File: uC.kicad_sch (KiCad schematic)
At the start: 21 parts, among them J7 Conn_01x03, P12 Conn_02x10_Odd_Even, SW1 SW_MEC_5E, SW2 SW_MEC_5E, U1 RPi-Pico

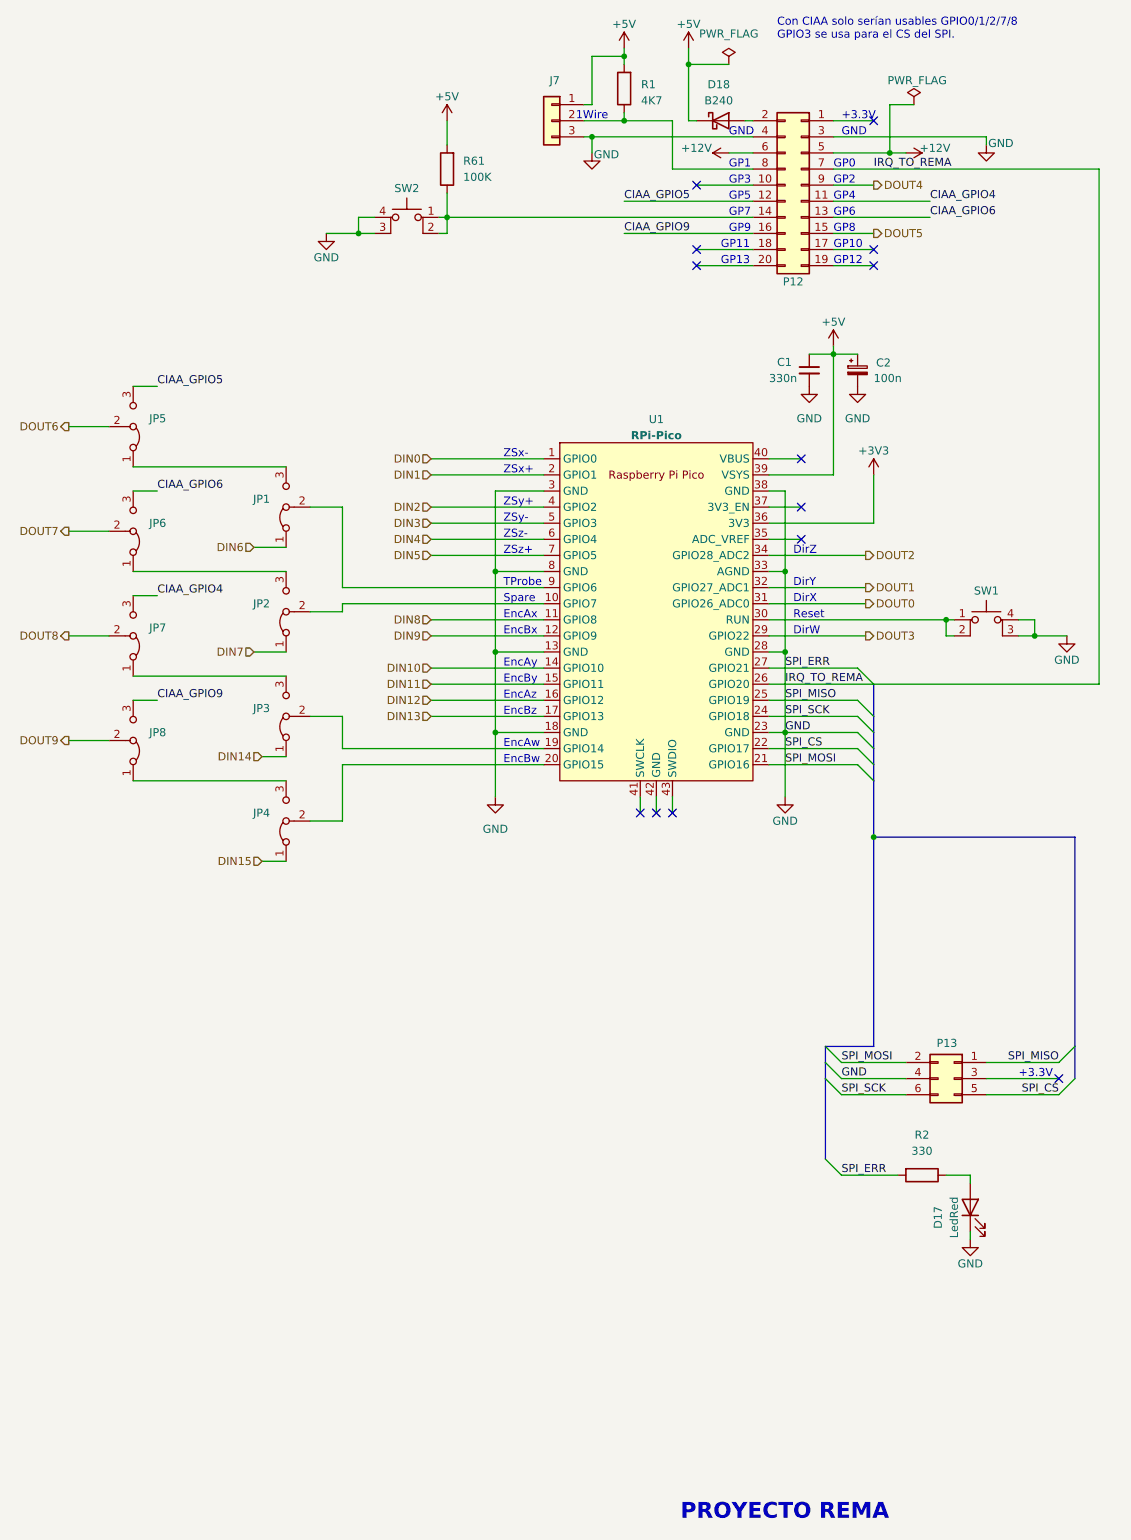
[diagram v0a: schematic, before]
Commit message: Comienza el diseño del pcb
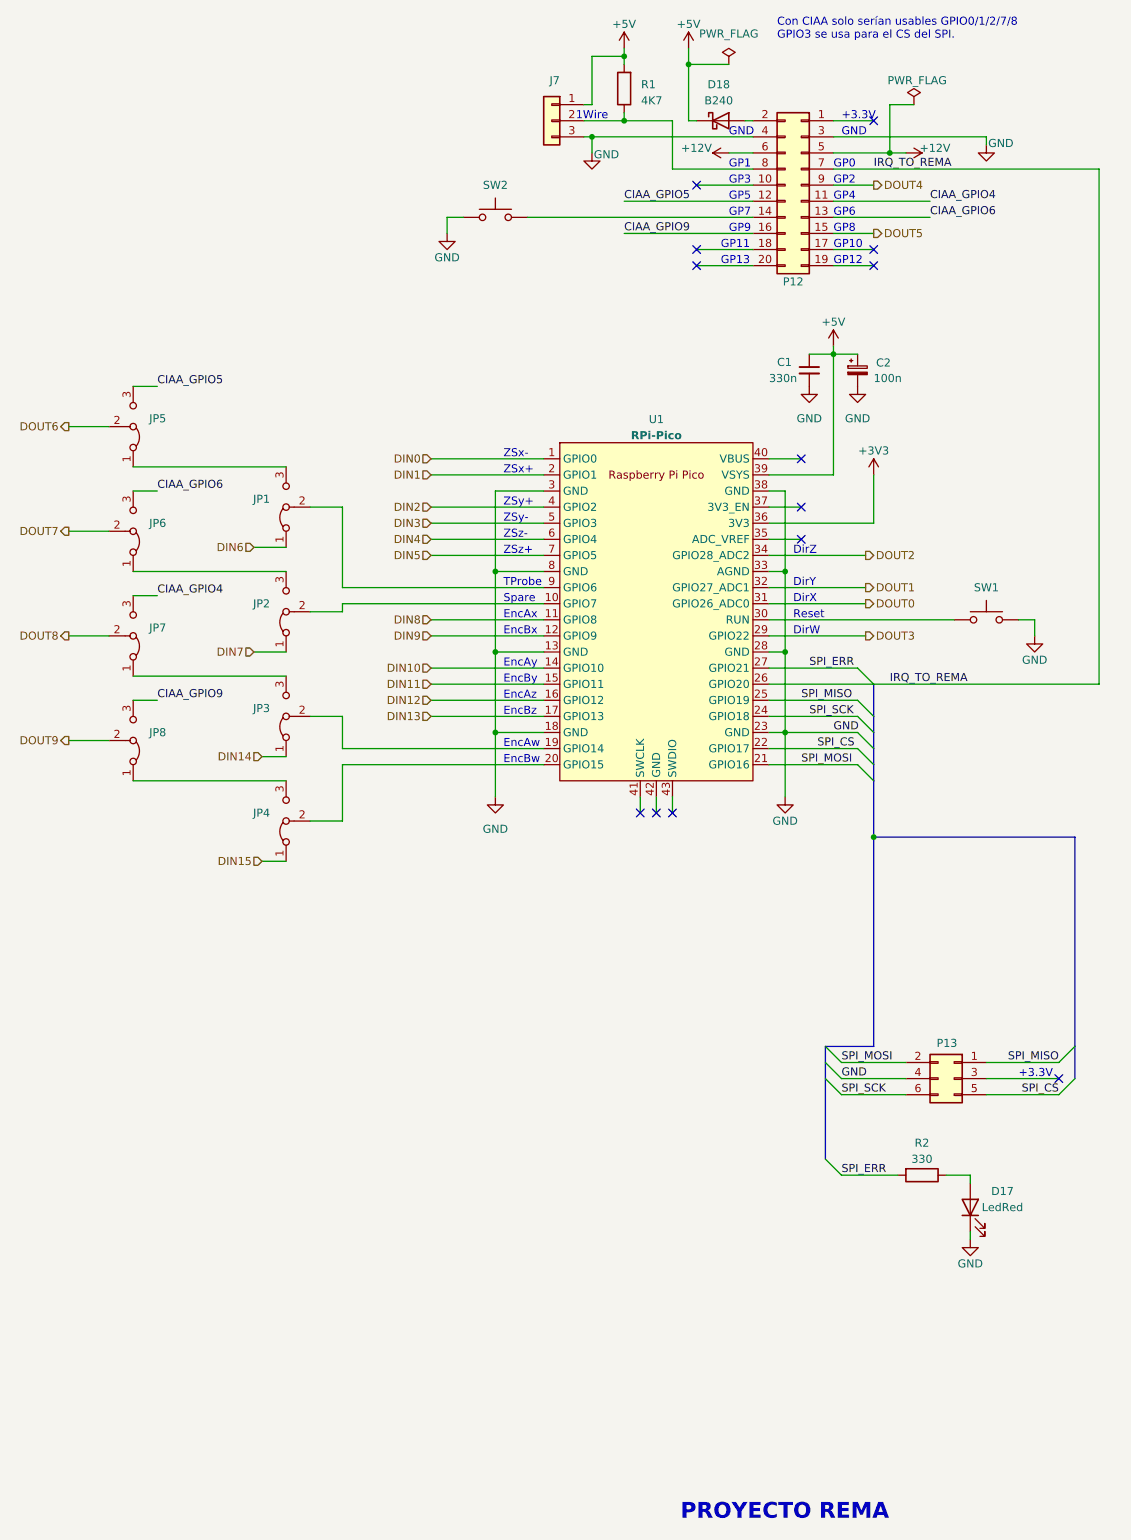
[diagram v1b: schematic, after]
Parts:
- removed R61: 100K, Resistor_SMD:R_1206_3216Metric, symbol Device:R
- removed SW1, SW2: SW_MEC_5E, Button_Switch_SMD:SW_Push_1P1T_NO_CK_KSC7xxJ, symbol Switch:SW_MEC_5E
- added SW1, SW2: SW_Push, Button_Switch_SMD:SW_Push_1P1T_NO_CK_KSC7xxJ, symbol Switch:SW_Push
- J7: footprint Connector_PinHeader_2.54mm:PinHeader_1x05_P2.54mm_Vertical -> Connector_PinHeader_2.54mm:PinHeader_1x03_P2.54mm_Vertical
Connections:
- net GND: now also SW1.2, SW2.1; no longer P12.7 (Pin_7), P13.1 (Pin_1), P13.2 (Pin_2), P13.5 (Pin_5), P13.6 (Pin_6), R2.2, U1.21 (GPIO16), U1.22 (GPIO17), U1.24 (GPIO18), U1.25 (GPIO19), U1.26 (GPIO20), U1.27 (GPIO21)
- net at U1.30 (RUN): now also SW1.1
- net at P12.14 (Pin_14): now also SW2.2
- new net IRQ_TO_REMA: P12.7 (Pin_7), U1.26 (GPIO20)
- new net SPI_CS: P13.5 (Pin_5), U1.22 (GPIO17)
- new net SPI_ERR: R2.2, U1.27 (GPIO21)
- new net SPI_MISO: P13.1 (Pin_1), U1.25 (GPIO19)
- new net SPI_MOSI: P13.2 (Pin_2), U1.21 (GPIO16)
- new net SPI_SCK: P13.6 (Pin_6), U1.24 (GPIO18)
